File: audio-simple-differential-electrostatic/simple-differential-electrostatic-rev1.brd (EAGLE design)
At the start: 152.4 x 139.7 mm, 73 parts, among them IC1 LT1115, IC2 LT1115, IC3 LT1115, IC4 LT1115, IC5 LM7815, IC7 LM317T, IC8 LM317T, IC9 LM7915, J1 ROUT, J2 LOUT, J3 VIN_PLATE, X1 RIN, X2 LIN, X3 VIN_OPAMP, X4 VIN_HEATER

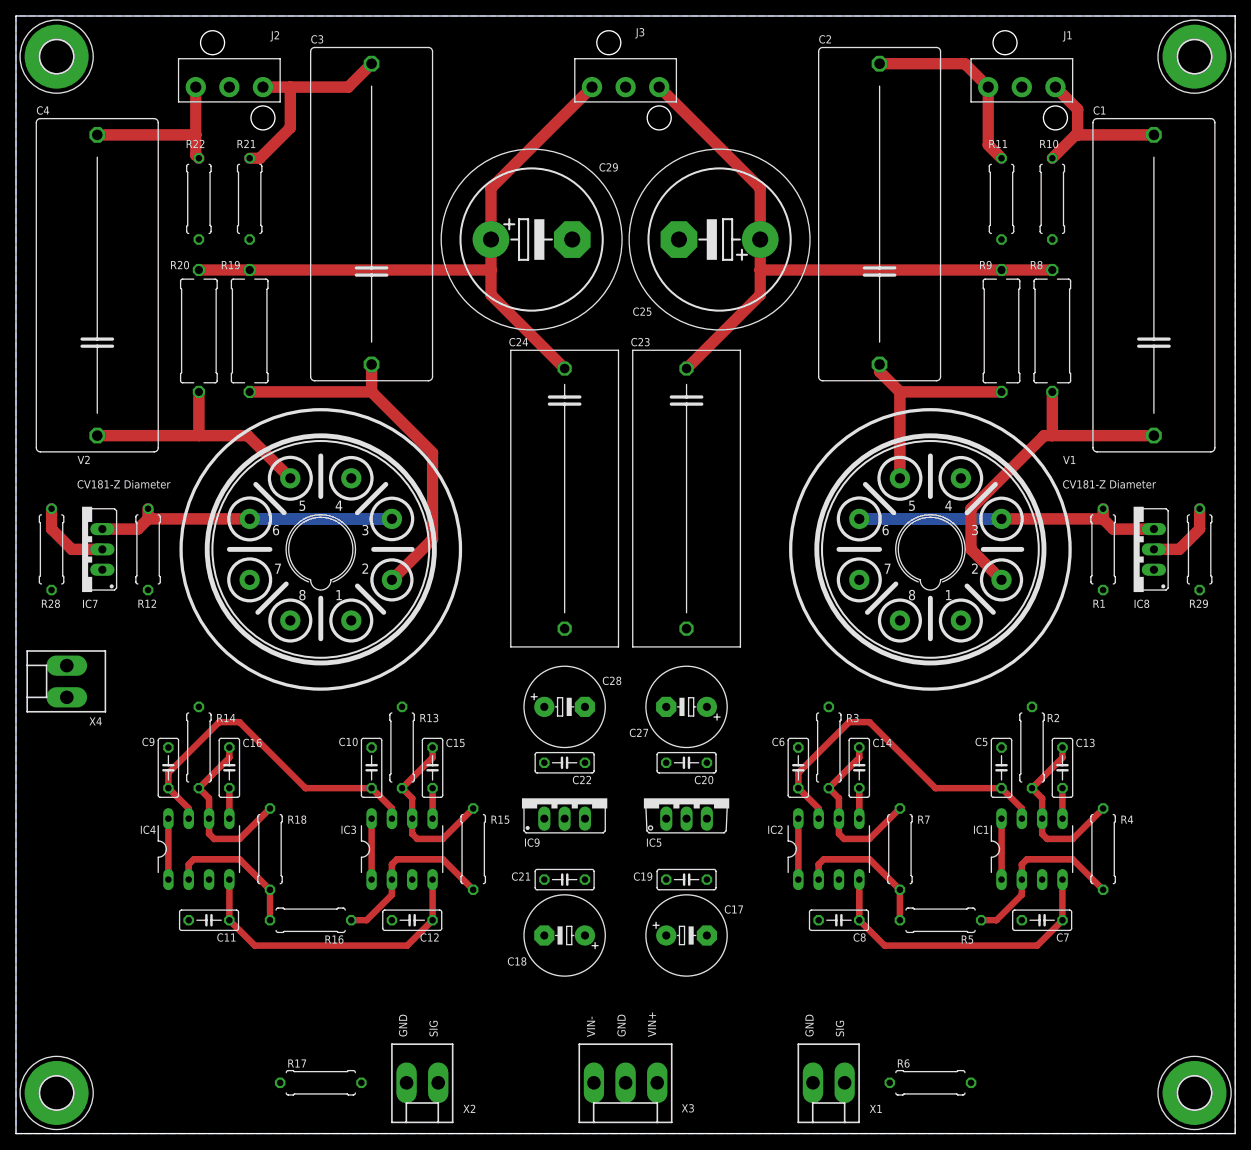
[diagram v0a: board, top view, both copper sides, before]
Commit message: First gerber export
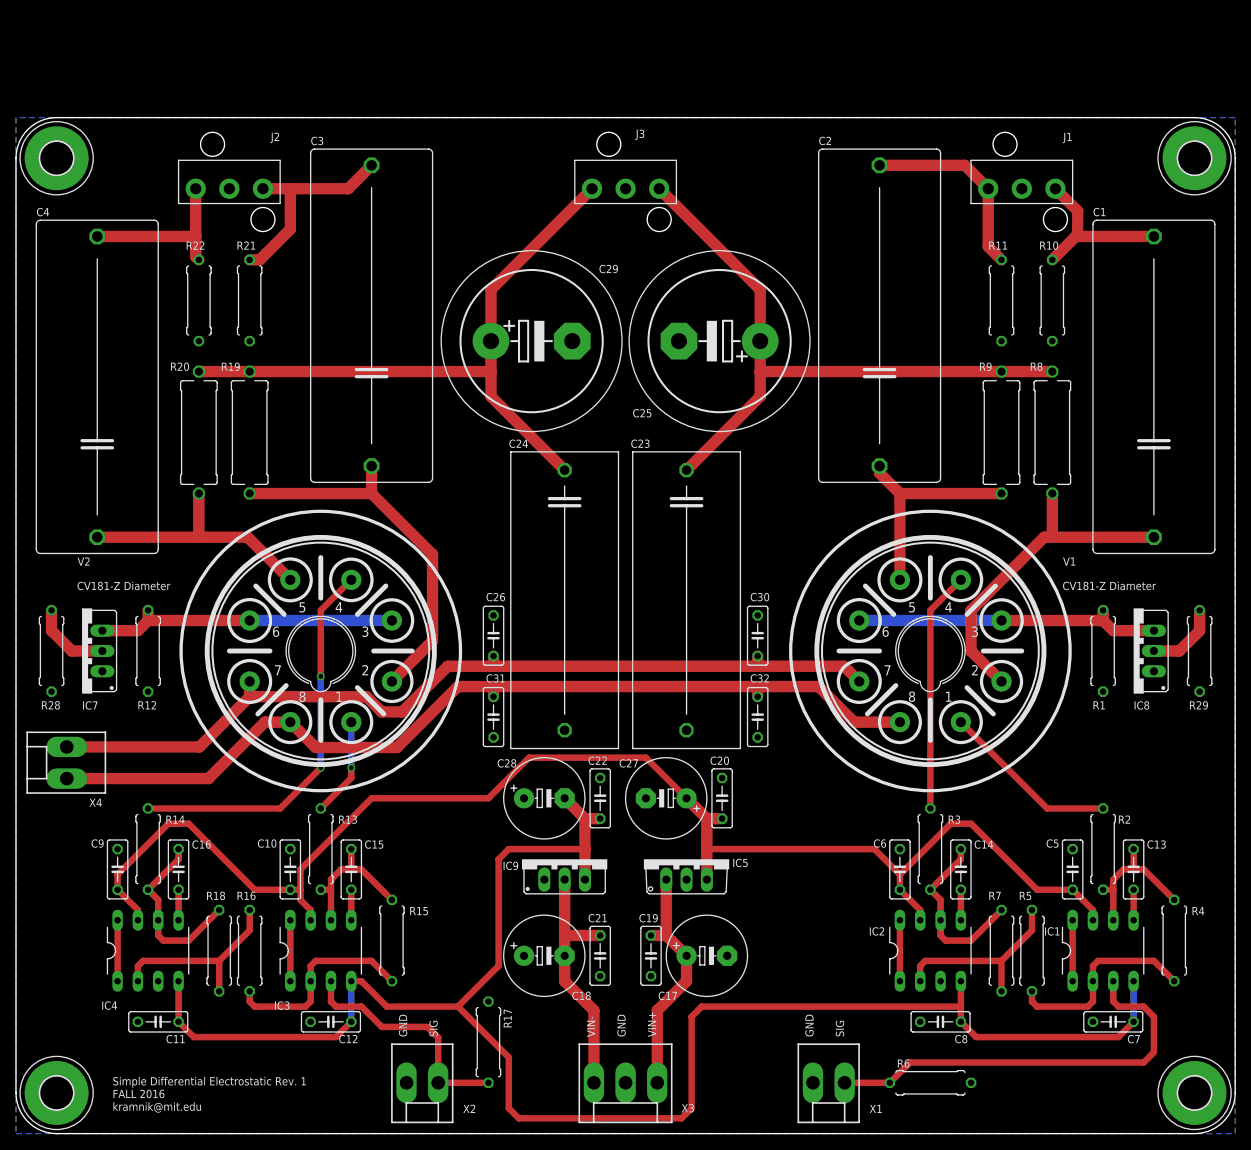
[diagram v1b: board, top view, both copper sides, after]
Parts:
- added C26, C30, C31, C32: 10n, rcl:C050-025X075
- moved R17 21.6 mm to (59.1, 11.4), turned to 270 degrees
- moved IC2 18.0 mm to (114.3, 22.9)
- moved R7 18.0 mm to (123.2, 22.9)
- moved C14 18.0 mm to (118.1, 33.0)
- moved R3 18.0 mm to (114.3, 35.6)
- moved C8 18.0 mm to (115.6, 14.0)
- moved C6 18.0 mm to (110.5, 33.0)
- moved C12 16.3 mm to (39.4, 14.0)
- moved C10 16.3 mm to (34.3, 33.0)
- moved C15 16.3 mm to (41.9, 33.0)
- moved IC3 16.3 mm to (38.1, 22.9)
- moved R13 16.3 mm to (38.1, 35.6)
- moved C5 15.5 mm to (132.1, 33.0)
- moved IC1 15.5 mm to (135.9, 22.9)
- moved C7 15.5 mm to (137.2, 14.0)
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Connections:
- net GND: now also C26.2, C30.2, C31.2, C32.2; no longer H1.B4,1, H2.B4,1, H3.B4,1, H4.B4,1
- net PP_HEATER_N: now also C31.1, C32.1
- net PP_HEATER_P: now also C26.1, C30.1
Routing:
- net PP_N15V0_OPAMP: track 76.4 -> 211.1 mm
- net PP_HEATER_N: track 0.00 -> 115.9 mm
- net PP_HEATER_P: track 0.00 -> 110.0 mm
- net PP_P15V0_OPAMP: track 86.2 -> 176.5 mm
- net R_INPUT: track 0.00 -> 53.1 mm
- net N$15: track 0.00 -> 48.8 mm, vias 0 -> 2
- net N$28: track 0.00 -> 31.4 mm
- net N$7: track 0.00 -> 30.2 mm
- net N$30: track 0.00 -> 29.9 mm
- net L_INPUT: track 0.00 -> 29.7 mm
- net N$8: track 0.00 -> 22.3 mm
- net N$16: track 0.00 -> 12.4 mm, vias 0 -> 1
- net N$21: track 17.7 -> 24.1 mm
- net N$13: track 17.7 -> 24.1 mm
- net N$17: track 22.4 -> 18.6 mm
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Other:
- board size 152.4 x 139.7 mm -> 152.4 x 127 mm
- board text added: "FALL 2016"
- board text added: "Simple Differential Electrostatic Rev. 1"
- board text added: "kramnik@mit.edu"
